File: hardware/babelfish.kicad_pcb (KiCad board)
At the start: 4 copper layers, 76 x 45.2 mm, 103 parts, among them J2 SWD, J3 DE9 Female, J4 USB_A, Q1 BSS138, SW1 TS342A2P-WZ, SW2 TS342A2P-WZ, U1 RP2040, U11 MAX3232IDR, U12 AP2191WG-7, U2 TPS2113ADRBR, U3 GT-USB-7010ASV, U36 TPS62933, U4 W25Q128JVS, U6 TPMCP1703T-3302E_CB, U7 74HC4052PW,118, U8 74HC4052PW,118, X1 X322512MSB4SI

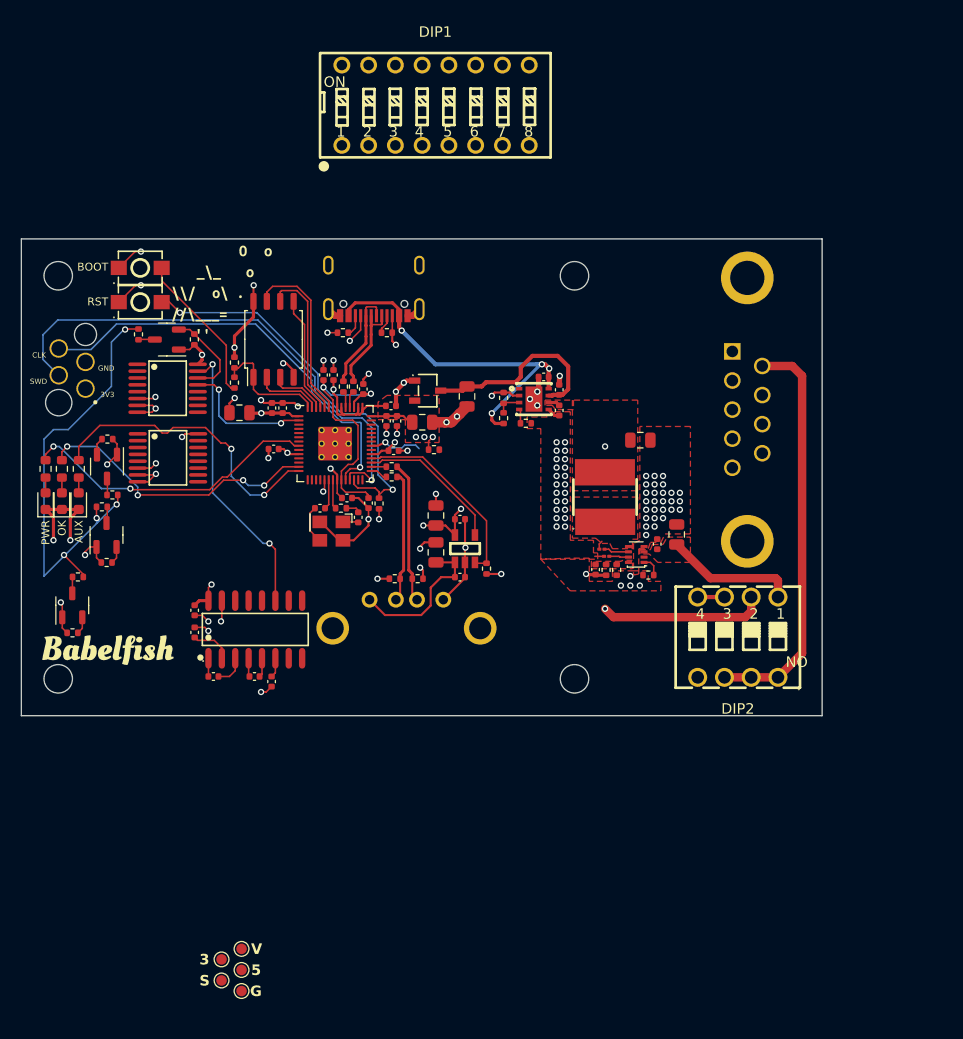
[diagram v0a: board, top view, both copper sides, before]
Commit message: WIP dip switches
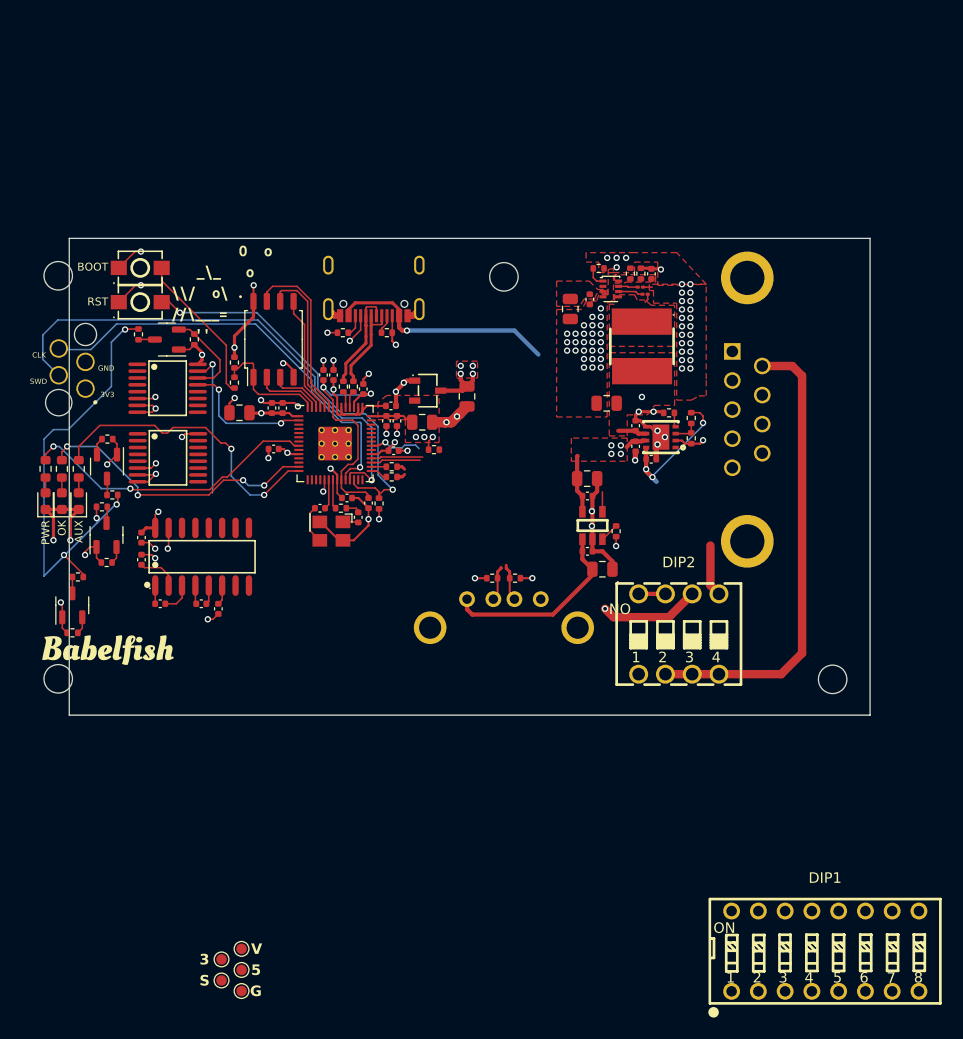
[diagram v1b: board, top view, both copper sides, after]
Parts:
- moved DIP1 88.4 mm to (93.5, 90.2)
- moved R37 29.5 mm to (72.0, 25.4), turned to 0 degrees
- moved C40 28.6 mm to (77.0, 25.9), turned to -90 degrees
- moved R36 28.3 mm to (76.0, 25.9), turned to -90 degrees
- moved R38 28.2 mm to (75.0, 25.9), turned to 90 degrees
- moved C39 25.7 mm to (76.0, 27.2), turned to 180 degrees
- moved U36 25.3 mm to (73.1, 27.4), turned to 0 degrees
- moved C36 24.5 mm to (76.4, 27.9), turned to 180 degrees
- moved H2 24.5 mm to (94.2, 64.4)
- moved C38 24.1 mm to (71.2, 28.3), turned to -90 degrees
- moved C37 23.7 mm to (69.3, 29.2), turned to -90 degrees
- moved R8 18.2 mm to (80.8, 41.5), turned to -90 degrees
- moved R6 17.8 mm to (80.8, 39.6), turned to -90 degrees
- moved C29 15.9 mm to (72.3, 54.0), turned to 0 degrees
- moved C31 14.8 mm to (70.9, 45.4), turned to 0 degrees
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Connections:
- DIP2 pad 1: /VCC_IN -> /VSHIFT
- DIP2 pad 2: /VCC_IN -> /VSHIFT
- DIP2 pad 3: /VCC_IN -> /VCC_5V
- DIP2 pad 4: /5V0 -> /VCC_IN_SW
- DIP2 pad 5: /VCC_IN_SW -> /5V0
- DIP2 pad 6: /VCC_5V -> /VCC_IN
- DIP2 pad 7: /VSHIFT -> /VCC_IN
- DIP2 pad 8: /VSHIFT -> /VCC_IN
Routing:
- net /TX_A_1Y2: track 26.9 -> 13.9 mm, vias 2 -> 1
- net /USB2_FLG: track 18.7 -> 6.76 mm
- net /5V0: track 24.8 -> 13.2 mm, vias 2 -> 8
- net /USB2_D+: track 13.4 -> 4.36 mm
- net /USB2_D-: track 13.1 -> 5.11 mm
- net /VCC_IN_SW: track 12.6 -> 4.93 mm
- net /USB2_EN: track 14.0 -> 6.63 mm
- net /VCC_IN: track 38.8 -> 44.3 mm
- net /VCC_5V: track 23.5 -> 18.9 mm
- net GND: track 109.5 -> 113.8 mm, vias 95 -> 96
- net /VBUS_OUT: track 14.4 -> 18.4 mm
- net VBUS: track 35.4 -> 36.5 mm
- net +3V3: track 56.4 -> 55.8 mm
- added copper zone on F.Cu, net /5V0
